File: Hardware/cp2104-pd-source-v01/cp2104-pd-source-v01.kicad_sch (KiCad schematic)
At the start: 1 part, among them U1 LDR6023C

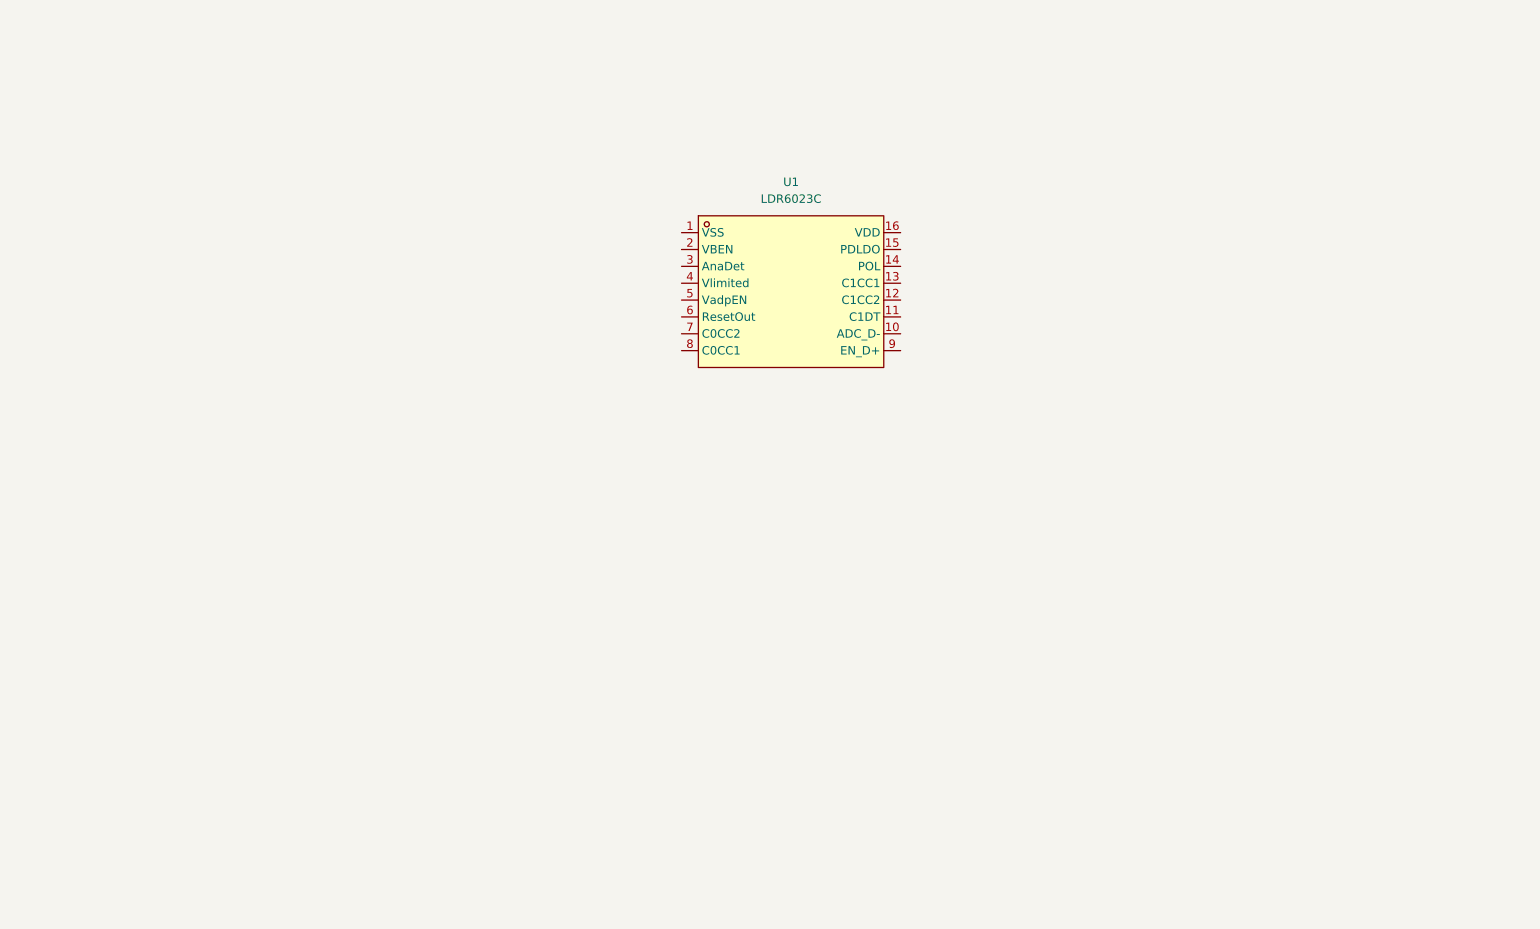
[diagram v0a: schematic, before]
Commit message: add final pcb
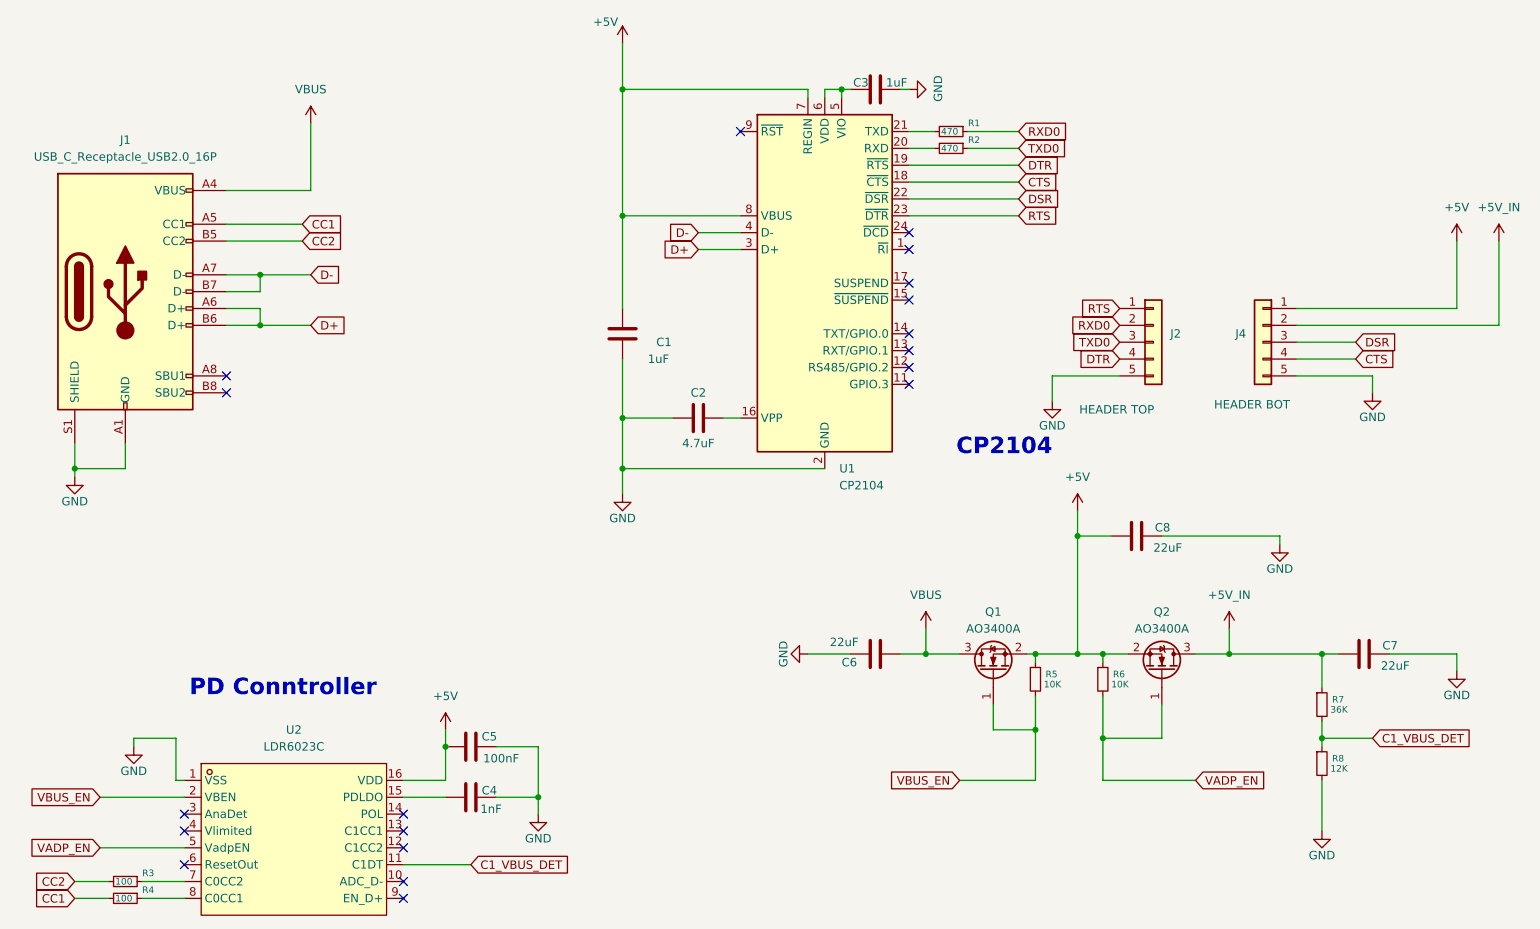
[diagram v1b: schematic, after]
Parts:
- removed U1: LDR6023C, easyeda2kicad:SSOP-16_L5.0-W4.4-P0.65-LS6.4-BL, symbol easyeda2kicad:LDR6023C
- added C1, C3: 1uF, Capacitor_SMD:C_0603_1608Metric, symbol Device:C
- added C2: 4.7uF, Capacitor_SMD:C_0603_1608Metric, symbol Device:C
- added C4: 1nF, Capacitor_SMD:C_0603_1608Metric, symbol Device:C
- added C5: 100nF, Capacitor_SMD:C_0603_1608Metric, symbol Device:C
- added C6, C7, C8: 22uF, Capacitor_SMD:C_1206_3216Metric, symbol Device:C
- added J1: USB_C_Receptacle_USB2.0_16P, Connector_USB:USB_C_Receptacle_GCT_USB4105-xx-A_16P_TopMnt_Horizontal, symbol Connector:USB_C_Receptacle_USB2.0_16P
- added J2: HEADER TOP, Connector_Harwin:Harwin_M20-89005xx_1x05_P2.54mm_Horizontal, symbol Connector_Generic:Conn_01x05
- added J4: HEADER BOT, Connector_Harwin:Harwin_M20-89005xx_1x05_P2.54mm_Horizontal, symbol Connector_Generic:Conn_01x05
- added Q1, Q2: AO3400A, Package_TO_SOT_SMD:SOT-23, symbol Transistor_FET:AO3400A
- added R1, R2: 470, Resistor_SMD:R_0603_1608Metric, symbol Device:R_Small
- added R3, R4: 100, Resistor_SMD:R_0603_1608Metric, symbol Device:R_Small
- added R5, R6: 10K, Resistor_SMD:R_0603_1608Metric, symbol Device:R_Small
- added R7: 36K, Resistor_SMD:R_0603_1608Metric, symbol Device:R_Small
- added R8: 12K, Resistor_SMD:R_0603_1608Metric, symbol Device:R_Small
- added U1: CP2104, Package_DFN_QFN:QFN-24-1EP_4x4mm_P0.5mm_EP2.6x2.6mm, symbol Interface_USB:CP2104
- added U2: LDR6023C, easyeda2kicad:SSOP-16_L5.0-W4.4-P0.65-LS6.4-BL, symbol easyeda2kicad:LDR6023C
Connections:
- new net: R2.2, U1.20 (RXD)
- new net: C4.1, U2.15 (PDLDO)
- new net: R3.1, U2.7 (C0CC2)
- new net: R4.1, U2.8 (C0CC1)
- new net: C3.1, U1.5 (VIO), U1.6 (VDD)
- new net: C2.1, U1.16 (VPP)
- new net: R1.2, U1.21 (TXD)
- new net +5V: C1.1, C5.1, C8.1, J4.1 (Pin_1), Q1.2 (S), Q2.2 (S), R5.1, R6.1, U1.7 (REGIN), U1.8 (VBUS), U2.16 (VDD)
- new net +5V_IN: C7.1, J4.2 (Pin_2), Q2.3 (D), R7.1
- new net C1_VBUS_DET: R7.2, R8.1, U2.11 (C1DT)
- new net CC1: J1.A5 (CC1), R4.2
- new net CC2: J1.B5 (CC2), R3.2
- new net CTS: J4.4 (Pin_4), U1.18 (~{CTS})
- new net D+: J1.A6 (D+), J1.B6 (D+), U1.3 (D+)
- new net D-: J1.A7 (D-), J1.B7 (D-), U1.4 (D-)
- new net DSR: J4.3 (Pin_3), U1.22 (~{DSR})
- new net DTR: J2.4 (Pin_4), U1.19 (~{RTS})
- new net GND: C1.2, C2.2, C3.2, C4.2, C5.2, C6.2, C7.2, C8.2, J1.A1 (GND), J1.A12 (GND), J1.B1 (GND), J1.B12 (GND), J1.S1 (SHIELD), J2.5 (Pin_5), J4.5 (Pin_5), R8.2, U1.2 (GND), U1.25 (GND), U2.1 (VSS)
- new net RTS: J2.1 (Pin_1), U1.23 (~{DTR})
- new net RXD0: J2.2 (Pin_2), R1.1
- new net TXD0: J2.3 (Pin_3), R2.1
- new net VADP_EN: Q2.1 (G), R6.2, U2.5 (VadpEN)
- new net VBUS: C6.1, J1.A4 (VBUS), J1.A9 (VBUS), J1.B4 (VBUS), J1.B9 (VBUS), Q1.3 (D)
- new net VBUS_EN: Q1.1 (G), R5.2, U2.2 (VBEN)
- no-connect marks 0 -> 19
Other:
- note added: "CP2104"
- note added: "PD Conntroller"
